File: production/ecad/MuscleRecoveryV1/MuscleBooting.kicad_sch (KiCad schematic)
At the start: 22 parts, among them J4 USB_C_Receptacle_USB2.0, Q2 AO3400A, Q3 AO3400A, SW1 SW_Push, SW2 SW_Push, U3 CP2102N-Axx-xQFN28

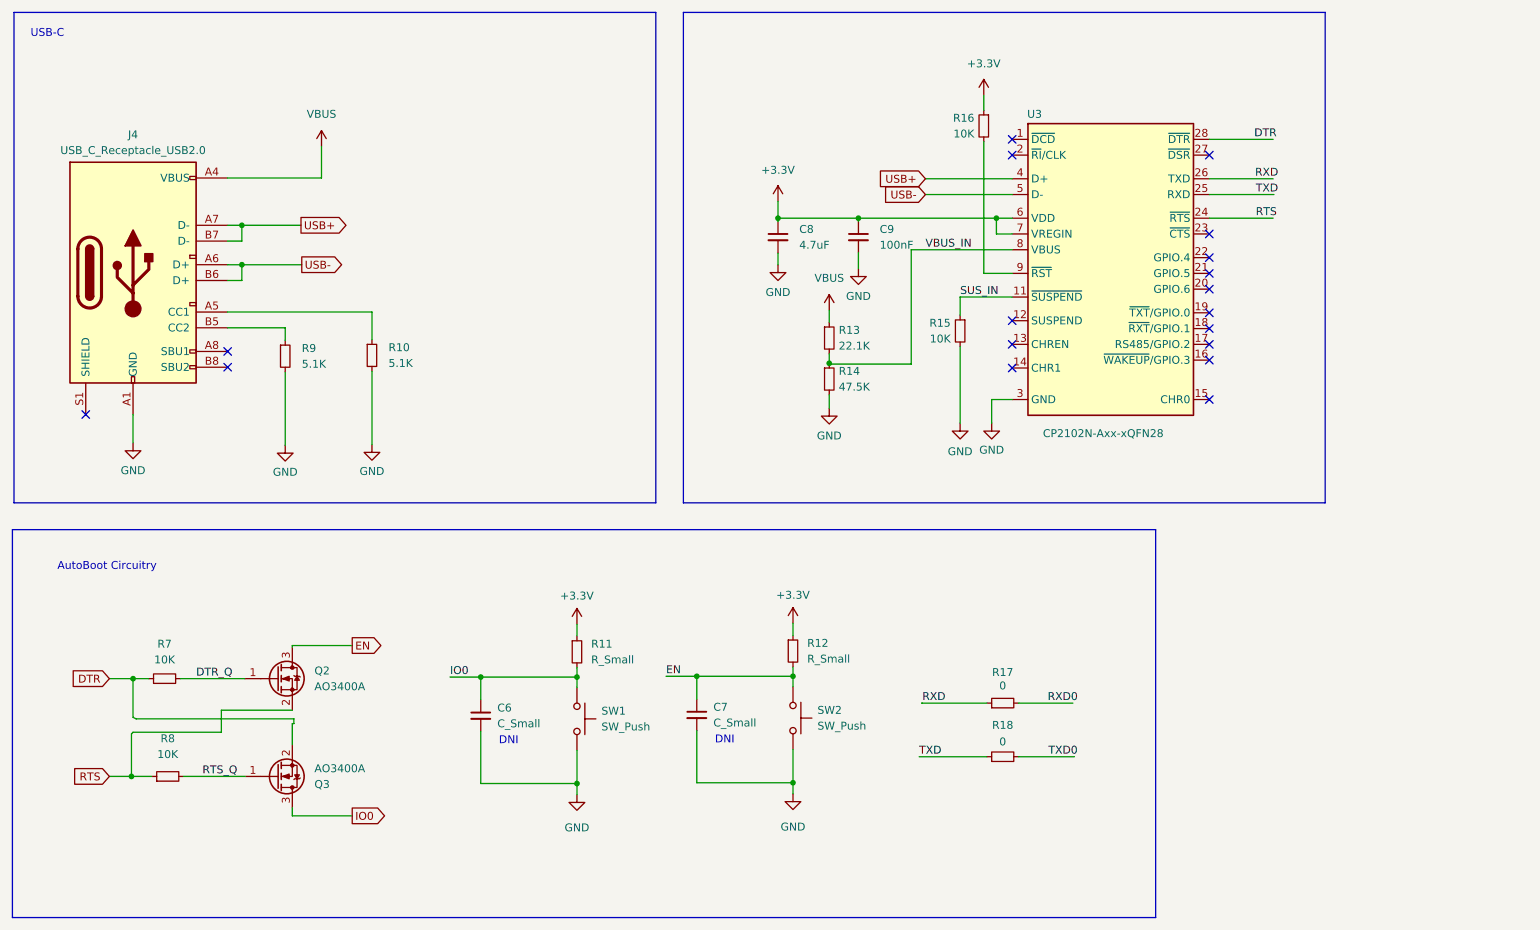
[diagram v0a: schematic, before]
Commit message: Revert "Display commit 1"
This reverts commit 52e50f7827ccbfa861bea7a8a003d131d02fed89.
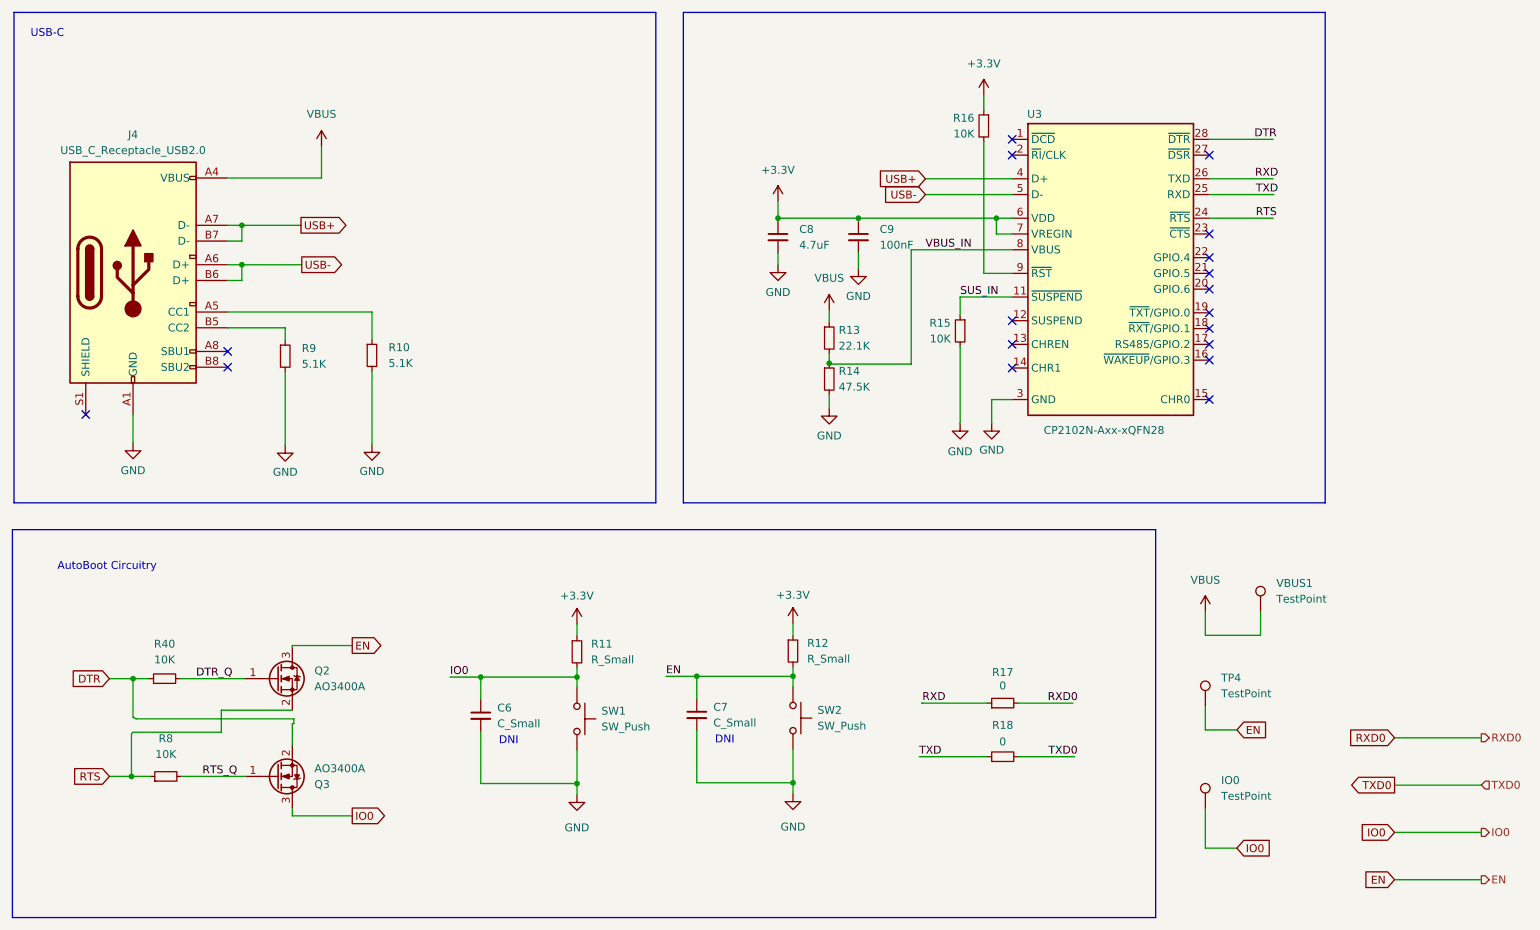
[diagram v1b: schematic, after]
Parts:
- removed R7: 10K, symbol Device:R_Small
- added IO0, TP4, VBUS1: TestPoint, symbol Connector:TestPoint
- added R40: 10K, symbol Device:R_Small
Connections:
- net DTR: now also R40.1
- net DTR_Q: now also R40.2
- net EN: now also TP4.1
- net GND: now also U3.29 (GND)
- net IO0: now also IO0.1
- net VBUS: now also VBUS1.1

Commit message: Display commit 1
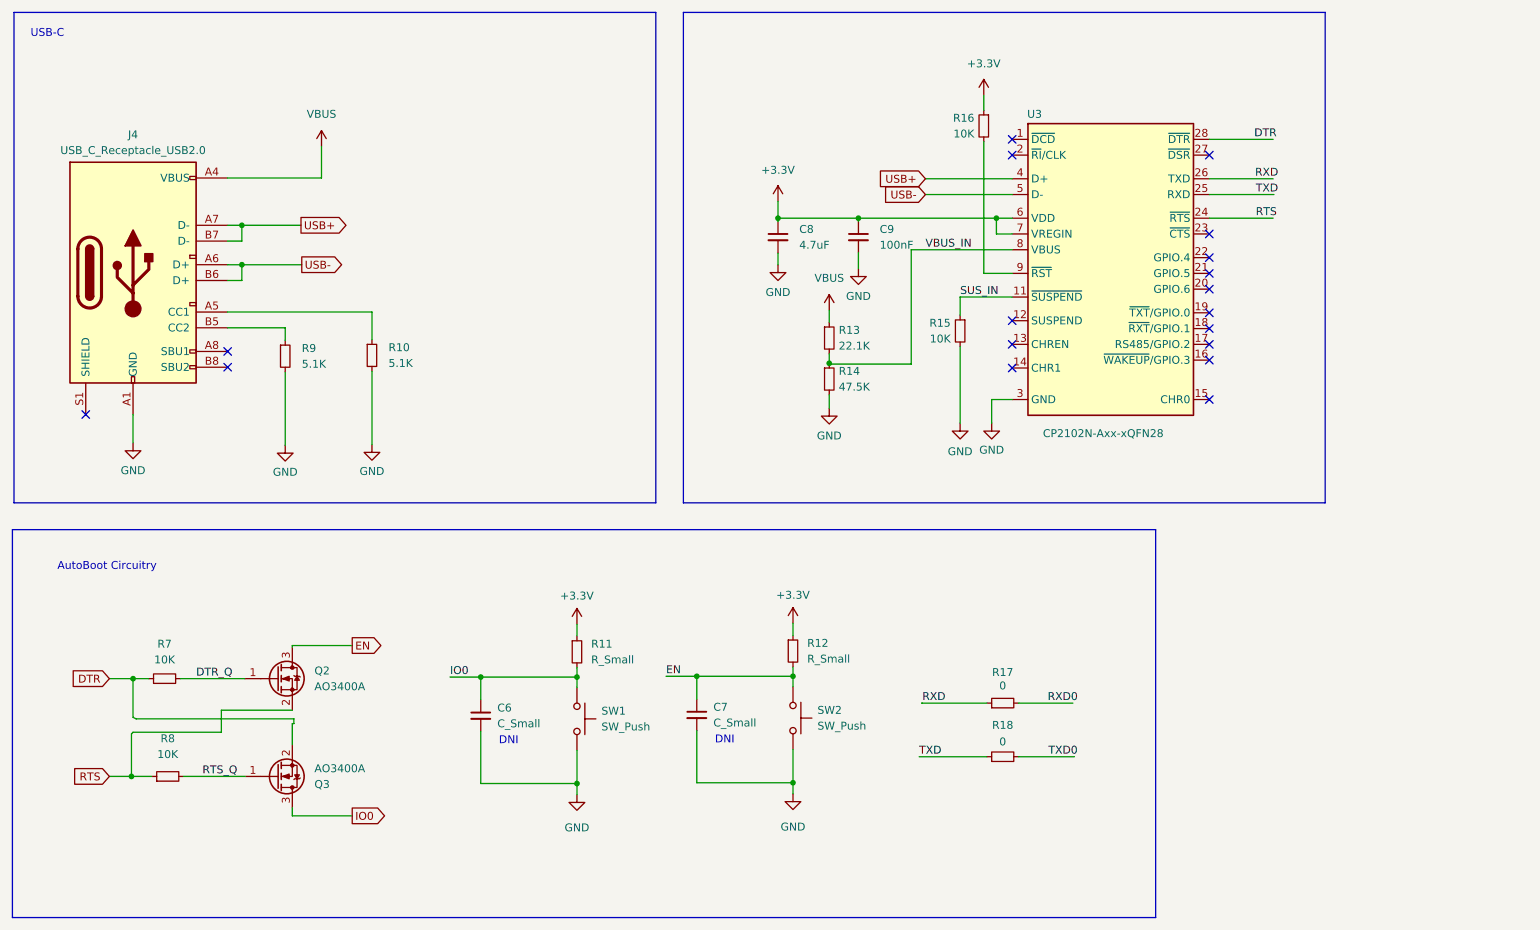
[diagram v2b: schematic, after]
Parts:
- removed IO0, TP4, VBUS1: TestPoint, symbol Connector:TestPoint
- removed R40: 10K, symbol Device:R_Small
- added R7: 10K, symbol Device:R_Small
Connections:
- net DTR: now also R7.1
- net DTR_Q: now also R7.2
- net GND: no longer U3.29 (GND)
